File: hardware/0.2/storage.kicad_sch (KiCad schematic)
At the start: 8 parts, among them J1 Micro_SD_Card, U7 S27KS0641

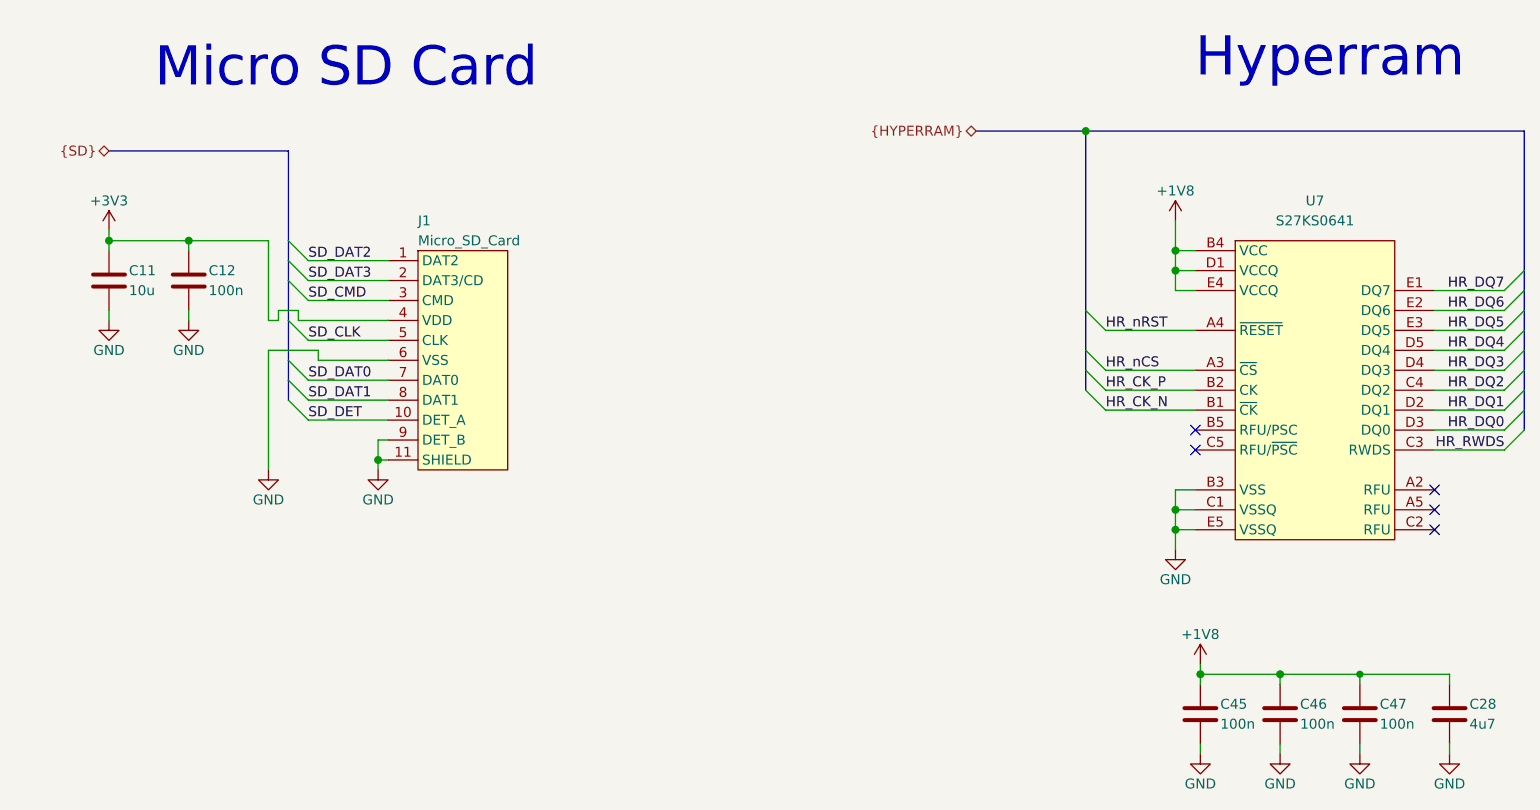
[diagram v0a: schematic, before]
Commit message: shipped 0.2
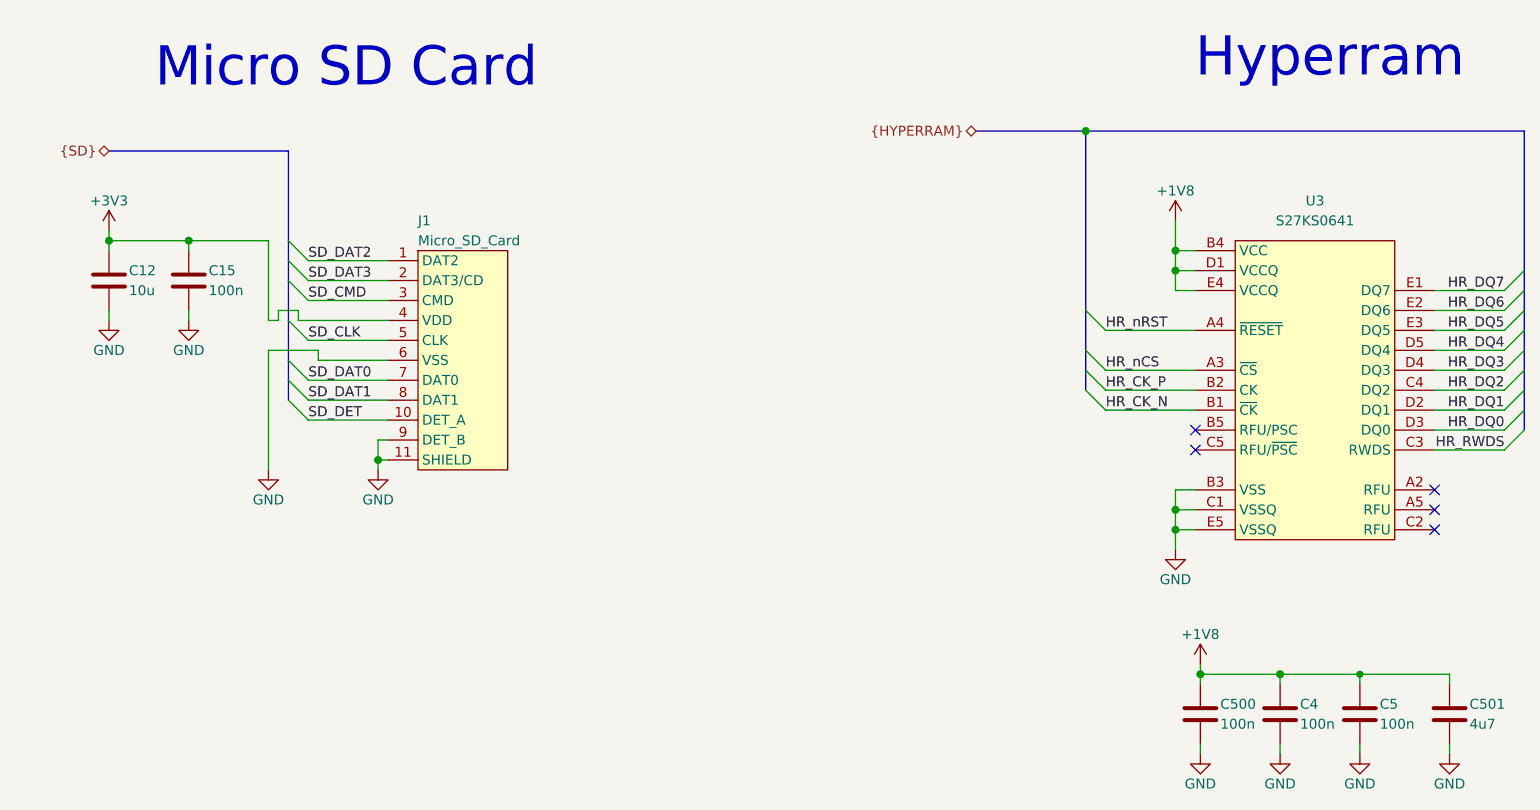
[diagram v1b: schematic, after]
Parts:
- C12: renamed from C11; LCSC C92487 -> C109453; MPN CL10A106MO8NQNC -> CC0603MRX5R6BB106; MPN2 (none) -> CL10A106KP8NNNC; Manufacturer Samsung Electro-Mechanics -> Yageo; Manufacturer2 (none) -> Samsung Electro-Mechanics
- C15: renamed from C12; LCSC C1525 -> C327009; MPN CL05B104KO5NNNC -> CC0402KRX7R7BB103; MPN2 (none) -> CL05B104KO5NNNC; Manufacturer Samsung Electro-Mechanics -> Yageo; Manufacturer2 (none) -> Samsung Electro-Mechanics
- C4: renamed from C46; LCSC C1525 -> C327009; MPN CL05B104KO5NNNC -> CC0402KRX7R7BB103; MPN2 (none) -> CL05B104KO5NNNC; Manufacturer Samsung Electro-Mechanics -> Yageo; Manufacturer2 (none) -> Samsung Electro-Mechanics
- C5: renamed from C47; LCSC C1525 -> C327009; MPN CL05B104KO5NNNC -> CC0402KRX7R7BB103; MPN2 (none) -> CL05B104KO5NNNC; Manufacturer Samsung Electro-Mechanics -> Yageo; Manufacturer2 (none) -> Samsung Electro-Mechanics
- C500: renamed from C45; LCSC C1525 -> C327009; MPN CL05B104KO5NNNC -> CC0402KRX7R7BB103; MPN2 (none) -> CL05B104KO5NNNC; Manufacturer Samsung Electro-Mechanics -> Yageo; Manufacturer2 (none) -> Samsung Electro-Mechanics
- C501: renamed from C28; LCSC C318563 -> C326586; MPN CL05A475MO5NUNC -> CC0402KRX5R6BB475; MPN2 (none) -> CL05A475KP5NRNC; Manufacturer Samsung Electro-Mechanics -> Yageo; Manufacturer2 (none) -> Samsung Electro-Mechanics
- U3: renamed from U7; MPN S27KS0641 -> S27KS0641DPBHI023; MPN2 (none) -> IS66WVH8M8ALL-166B1LI; Manufacturer2 (none) -> ISSI
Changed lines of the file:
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@@
   (title_block
     (title "ECP5 Mini")
-    (date "2020-12-27")
+    (date "2020-12-31")
     (rev "0.2")
     (company "Josh Johnson")
@@
   (junction (at 219.075 128.905) (diameter 0.9144) (color 0 0 0 0))
   (junction (at 184.15 59.69) (diameter 1.016) (color 0 0 0 0))
+  (no_connect (at 198.12 100.33))
   (no_connect (at 198.12 97.79))
-  (no_connect (at 198.12 100.33))
+  (no_connect (at 228.6 107.95))
+  (no_connect (at 228.6 110.49))
   (no_connect (at 228.6 105.41))
-  (no_connect (at 228.6 110.49))
-  (no_connect (at 228.6 107.95))
   (bus_entry (at 82.55 73.66) (size 2.54 2.54)
     (stroke (width 0.1524) (type solid) (color 0 0 0 0))
@@
   (symbol (lib_id "Device:C") (at 59.69 78.74 0) (unit 1)
     (in_bom yes) (on_board yes)
-    (property "Reference" "C11" (id 0) (at 62.23 77.47 0)
+    (property "Reference" "C12" (id 0) (at 62.23 77.47 0)
       (effects (font (size 1.27 1.27)) (justify left))
     )
@@
       (effects (font (size 1.27 1.27)) hide)
     )
-    (property "LCSC" "C92487" (id 4) (at 59.69 78.74 0)
-      (effects (font (size 1.27 1.27)) hide)
-    )
-    (property "MPN" "CL10A106MO8NQNC" (id 5) (at 59.69 78.74 0)
-      (effects (font (size 1.27 1.27)) hide)
-    )
-    (property "Manufacturer" "Samsung Electro-Mechanics" (id 6) (at 59.69 78.74 0)
+    (property "LCSC" "C109453" (id 4) (at 59.69 78.74 0)
+      (effects (font (size 1.27 1.27)) hide)
+    )
+    (property "MPN" "CC0603MRX5R6BB106" (id 5) (at 59.69 78.74 0)
+      (effects (font (size 1.27 1.27)) hide)
+    )
+    (property "Manufacturer" "Yageo" (id 6) (at 59.69 78.74 0)
+      (effects (font (size 1.27 1.27)) hide)
+    )
+    (property "MPN2" "CL10A106KP8NNNC" (id 4) (at 59.69 78.74 0)
+      (effects (font (size 1.27 1.27)) hide)
+    )
+    (property "Manufacturer2" "Samsung Electro-Mechanics" (id 5) (at 59.69 78.74 0)
       (effects (font (size 1.27 1.27)) hide)
     )
@@
   (symbol (lib_id "Device:C") (at 69.85 78.74 0) (unit 1)
     (in_bom yes) (on_board yes)
-    (property "Reference" "C12" (id 0) (at 72.39 77.47 0)
+    (property "Reference" "C15" (id 0) (at 72.39 77.47 0)
       (effects (font (size 1.27 1.27)) (justify left))
     )
@@
       (effects (font (size 1.27 1.27)) hide)
     )
-    (property "LCSC" "C1525" (id 4) (at 69.85 78.74 0)
-      (effects (font (size 1.27 1.27)) hide)
-    )
-    (property "MPN" "CL05B104KO5NNNC" (id 5) (at 69.85 78.74 0)
-      (effects (font (size 1.27 1.27)) hide)
-    )
-    (property "Manufacturer" "Samsung Electro-Mechanics" (id 6) (at 69.85 78.74 0)
+    (property "LCSC" "C327009" (id 4) (at 69.85 78.74 0)
+      (effects (font (size 1.27 1.27)) hide)
+    )
+    (property "MPN" "CC0402KRX7R7BB103" (id 5) (at 69.85 78.74 0)
+      (effects (font (size 1.27 1.27)) hide)
+    )
+    (property "Manufacturer" "Yageo" (id 6) (at 69.85 78.74 0)
+      (effects (font (size 1.27 1.27)) hide)
+    )
+    (property "MPN2" "CL05B104KO5NNNC" (id 4) (at 69.85 78.74 0)
+      (effects (font (size 1.27 1.27)) hide)
+    )
+    (property "Manufacturer2" "Samsung Electro-Mechanics" (id 5) (at 69.85 78.74 0)
       (effects (font (size 1.27 1.27)) hide)
     )
@@
   (symbol (lib_id "Device:C") (at 198.755 133.985 0) (unit 1)
     (in_bom yes) (on_board yes)
-    (property "Reference" "C45" (id 0) (at 201.295 132.715 0)
+    (property "Reference" "C500" (id 0) (at 201.295 132.715 0)
       (effects (font (size 1.27 1.27)) (justify left))
     )
@@
       (effects (font (size 1.27 1.27)) hide)
     )
-    (property "LCSC" "C1525" (id 4) (at 198.755 133.985 0)
-      (effects (font (size 1.27 1.27)) hide)
-    )
-    (property "MPN" "CL05B104KO5NNNC" (id 5) (at 198.755 133.985 0)
-      (effects (font (size 1.27 1.27)) hide)
-    )
-    (property "Manufacturer" "Samsung Electro-Mechanics" (id 6) (at 198.755 133.985 0)
+    (property "LCSC" "C327009" (id 4) (at 198.755 133.985 0)
+      (effects (font (size 1.27 1.27)) hide)
+    )
+    (property "MPN" "CC0402KRX7R7BB103" (id 5) (at 198.755 133.985 0)
+      (effects (font (size 1.27 1.27)) hide)
+    )
+    (property "Manufacturer" "Yageo" (id 6) (at 198.755 133.985 0)
+      (effects (font (size 1.27 1.27)) hide)
+    )
+    (property "MPN2" "CL05B104KO5NNNC" (id 4) (at 198.755 133.985 0)
+      (effects (font (size 1.27 1.27)) hide)
+    )
+    (property "Manufacturer2" "Samsung Electro-Mechanics" (id 5) (at 198.755 133.985 0)
       (effects (font (size 1.27 1.27)) hide)
     )
@@
   (symbol (lib_id "Device:C") (at 208.915 133.985 0) (unit 1)
     (in_bom yes) (on_board yes)
-    (property "Reference" "C46" (id 0) (at 211.455 132.715 0)
+    (property "Reference" "C4" (id 0) (at 211.455 132.715 0)
       (effects (font (size 1.27 1.27)) (justify left))
     )
@@
       (effects (font (size 1.27 1.27)) hide)
     )
-    (property "LCSC" "C1525" (id 4) (at 208.915 133.985 0)
-      (effects (font (size 1.27 1.27)) hide)
-    )
-    (property "MPN" "CL05B104KO5NNNC" (id 5) (at 208.915 133.985 0)
-      (effects (font (size 1.27 1.27)) hide)
-    )
-    (property "Manufacturer" "Samsung Electro-Mechanics" (id 6) (at 208.915 133.985 0)
+    (property "LCSC" "C327009" (id 4) (at 208.915 133.985 0)
+      (effects (font (size 1.27 1.27)) hide)
+    )
+    (property "MPN" "CC0402KRX7R7BB103" (id 5) (at 208.915 133.985 0)
+      (effects (font (size 1.27 1.27)) hide)
+    )
+    (property "Manufacturer" "Yageo" (id 6) (at 208.915 133.985 0)
+      (effects (font (size 1.27 1.27)) hide)
+    )
+    (property "MPN2" "CL05B104KO5NNNC" (id 4) (at 208.915 133.985 0)
+      (effects (font (size 1.27 1.27)) hide)
+    )
+    (property "Manufacturer2" "Samsung Electro-Mechanics" (id 5) (at 208.915 133.985 0)
       (effects (font (size 1.27 1.27)) hide)
     )
@@
   (symbol (lib_id "Device:C") (at 219.075 133.985 0) (unit 1)
     (in_bom yes) (on_board yes)
-    (property "Reference" "C47" (id 0) (at 221.615 132.715 0)
+    (property "Reference" "C5" (id 0) (at 221.615 132.715 0)
       (effects (font (size 1.27 1.27)) (justify left))
     )
@@
       (effects (font (size 1.27 1.27)) hide)
     )
-    (property "LCSC" "C1525" (id 4) (at 219.075 133.985 0)
-      (effects (font (size 1.27 1.27)) hide)
-    )
-    (property "MPN" "CL05B104KO5NNNC" (id 5) (at 219.075 133.985 0)
-      (effects (font (size 1.27 1.27)) hide)
-    )
-    (property "Manufacturer" "Samsung Electro-Mechanics" (id 6) (at 219.075 133.985 0)
+    (property "LCSC" "C327009" (id 4) (at 219.075 133.985 0)
+      (effects (font (size 1.27 1.27)) hide)
+    )
+    (property "MPN" "CC0402KRX7R7BB103" (id 5) (at 219.075 133.985 0)
+      (effects (font (size 1.27 1.27)) hide)
+    )
+    (property "Manufacturer" "Yageo" (id 6) (at 219.075 133.985 0)
+      (effects (font (size 1.27 1.27)) hide)
+    )
+    (property "MPN2" "CL05B104KO5NNNC" (id 4) (at 219.075 133.985 0)
+      (effects (font (size 1.27 1.27)) hide)
+    )
+    (property "Manufacturer2" "Samsung Electro-Mechanics" (id 5) (at 219.075 133.985 0)
       (effects (font (size 1.27 1.27)) hide)
     )
@@
   (symbol (lib_id "Device:C") (at 230.505 133.985 0) (unit 1)
     (in_bom yes) (on_board yes)
-    (property "Reference" "C28" (id 0) (at 233.045 132.715 0)
+    (property "Reference" "C501" (id 0) (at 233.045 132.715 0)
       (effects (font (size 1.27 1.27)) (justify left))
     )
@@
       (effects (font (size 1.27 1.27)) hide)
     )
-    (property "LCSC" "C318563" (id 4) (at 230.505 133.985 0)
-      (effects (font (size 1.27 1.27)) hide)
-    )
-    (property "MPN" "CL05A475MO5NUNC" (id 5) (at 230.505 133.985 0)
-      (effects (font (size 1.27 1.27)) hide)
-    )
-    (property "Manufacturer" "Samsung Electro-Mechanics" (id 6) (at 230.505 133.985 0)
+    (property "LCSC" "C326586" (id 4) (at 230.505 133.985 0)
+      (effects (font (size 1.27 1.27)) hide)
+    )
+    (property "MPN" "CC0402KRX5R6BB475" (id 5) (at 230.505 133.985 0)
+      (effects (font (size 1.27 1.27)) hide)
+    )
+    (property "Manufacturer" "Yageo" (id 6) (at 230.505 133.985 0)
+      (effects (font (size 1.27 1.27)) hide)
+    )
+    (property "MPN2" "CL05A475KP5NRNC" (id 4) (at 230.505 133.985 0)
+      (effects (font (size 1.27 1.27)) hide)
+    )
+    (property "Manufacturer2" "Samsung Electro-Mechanics" (id 5) (at 230.505 133.985 0)
       (effects (font (size 1.27 1.27)) hide)
     )
@@
       (effects (font (size 1.27 1.27)) hide)
     )
-    (property "Mouser" "" (id 6) (at 104.14 87.63 0)
-      (effects (font (size 1.27 1.27)) hide)
-    )
     (property "LCSC" "C585350" (id 4) (at 104.14 87.63 0)
       (effects (font (size 1.27 1.27)) hide)
@@
   (symbol (lib_id "josh-memory:S27KL0641") (at 213.36 92.71 0) (unit 1)
     (in_bom yes) (on_board yes)
-    (property "Reference" "U7" (id 0) (at 213.36 68.58 0))
+    (property "Reference" "U3" (id 0) (at 213.36 68.58 0))
     (property "Value" "S27KS0641" (id 1) (at 213.36 71.12 0))
     (property "Footprint" "josh-bga:BGA-24_5x5_6.0x8.0mm" (id 2) (at 228.6 115.57 0)
@@
       (effects (font (size 1.27 1.27)) hide)
     )
-    (property "MPN" "S27KS0641" (id 4) (at 213.36 92.71 0)
+    (property "MPN" "S27KS0641DPBHI023" (id 4) (at 213.36 92.71 0)
       (effects (font (size 1.27 1.27)) hide)
     )
@@
       (effects (font (size 1.27 1.27)) hide)
     )
-    (property "Mouser" "" (id 6) (at 213.36 92.71 0)
-      (effects (font (size 1.27 1.27)) hide)
-    )
+    (property "MPN2" "IS66WVH8M8ALL-166B1LI" (id 4) (at 213.36 92.71 0)
+      (effects (font (size 1.27 1.27)) hide)
+    )
+    (property "Manufacturer2" "ISSI" (id 5) (at 213.36 92.71 0)
+      (effects (font (size 1.27 1.27)) hide)
+    )

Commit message: bom fix
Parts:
- C15, C4, C5, C500: MPN CC0402KRX7R7BB103 -> CC0402KRX7R7BB104
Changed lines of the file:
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@@
   (junction (at 219.075 128.905) (diameter 0.9144) (color 0 0 0 0))
   (junction (at 184.15 59.69) (diameter 1.016) (color 0 0 0 0))
+  (no_connect (at 228.6 105.41))
+  (no_connect (at 198.12 100.33))
   (no_connect (at 198.12 97.79))
-  (no_connect (at 228.6 105.41))
   (no_connect (at 228.6 107.95))
   (no_connect (at 228.6 110.49))
-  (no_connect (at 198.12 100.33))
   (bus_entry (at 82.55 73.66) (size 2.54 2.54)
     (stroke (width 0.1524) (type solid) (color 0 0 0 0))
@@
       (effects (font (size 1.27 1.27)) hide)
     )
-    (property "MPN" "CC0402KRX7R7BB103" (id 5) (at 69.85 78.74 0)
+    (property "MPN" "CC0402KRX7R7BB104" (id 5) (at 69.85 78.74 0)
       (effects (font (size 1.27 1.27)) hide)
     )
@@
       (effects (font (size 1.27 1.27)) hide)
     )
-    (property "MPN" "CC0402KRX7R7BB103" (id 5) (at 198.755 133.985 0)
+    (property "MPN" "CC0402KRX7R7BB104" (id 5) (at 198.755 133.985 0)
       (effects (font (size 1.27 1.27)) hide)
     )
@@
       (effects (font (size 1.27 1.27)) hide)
     )
-    (property "MPN" "CC0402KRX7R7BB103" (id 5) (at 208.915 133.985 0)
+    (property "MPN" "CC0402KRX7R7BB104" (id 5) (at 208.915 133.985 0)
       (effects (font (size 1.27 1.27)) hide)
     )
@@
       (effects (font (size 1.27 1.27)) hide)
     )
-    (property "MPN" "CC0402KRX7R7BB103" (id 5) (at 219.075 133.985 0)
-      (effects (font (size 1.27 1.27)) hide)
-    )
+    (property "MPN" "CC0402KRX7R7BB104" (id 5) (at 219.075 133.985 0)
+      (effects (font (size 1.27 1.27)) hide)
+    )
